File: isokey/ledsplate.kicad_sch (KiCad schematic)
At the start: 143 parts

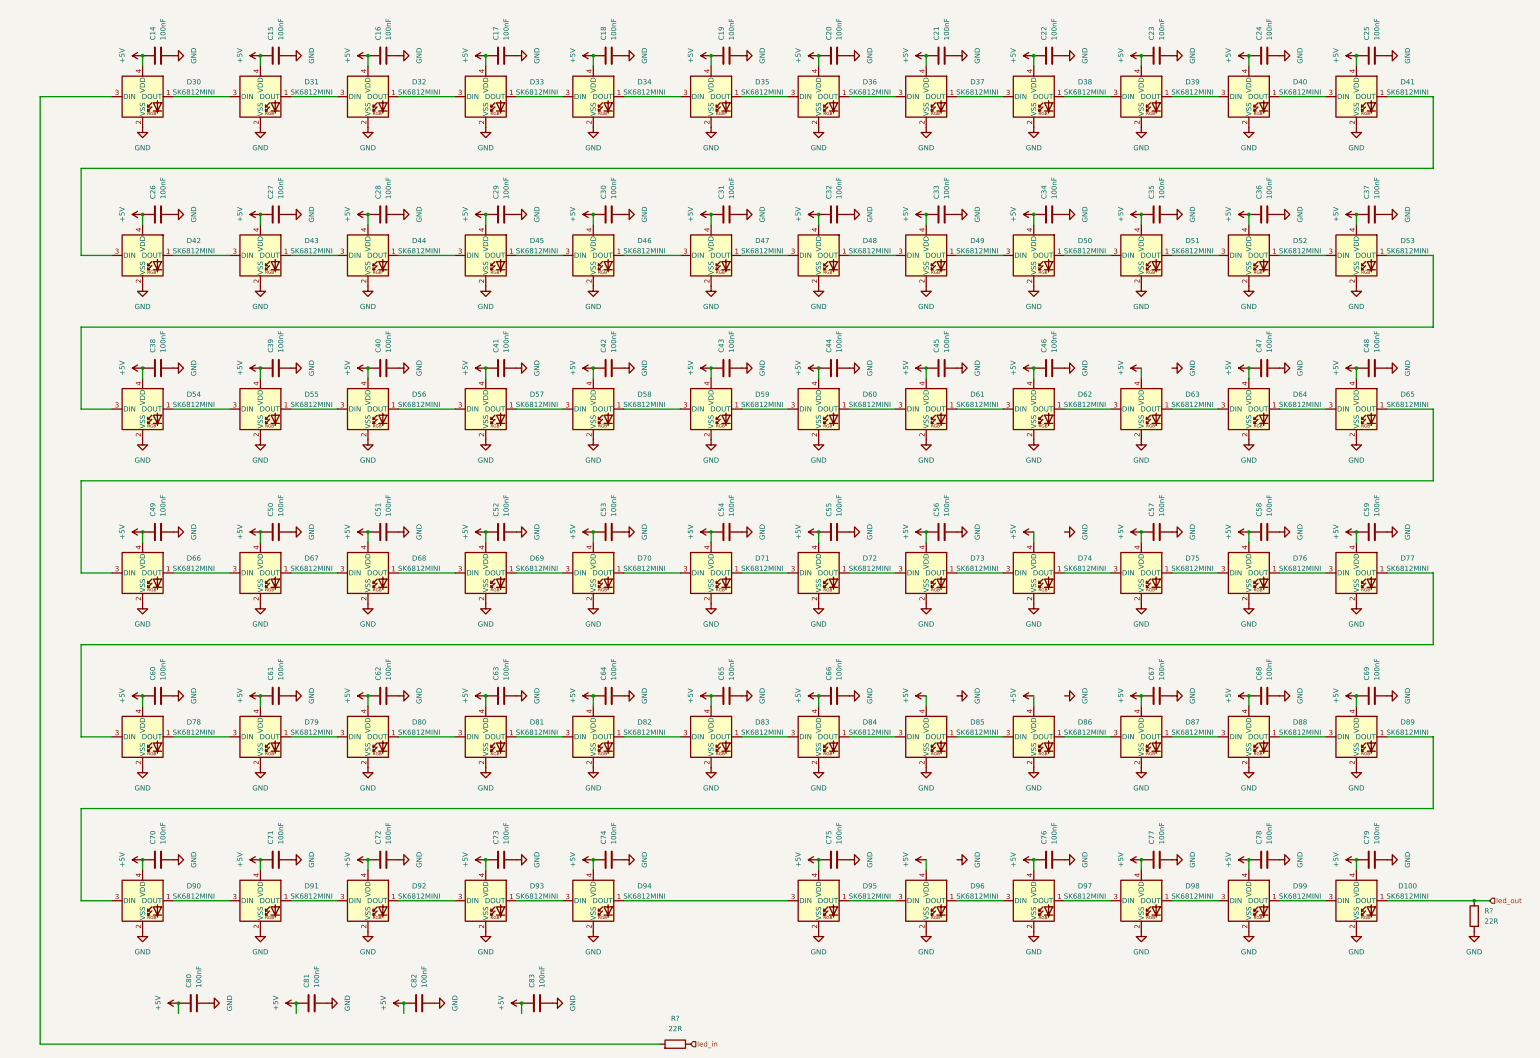
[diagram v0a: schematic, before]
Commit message: Continue routing
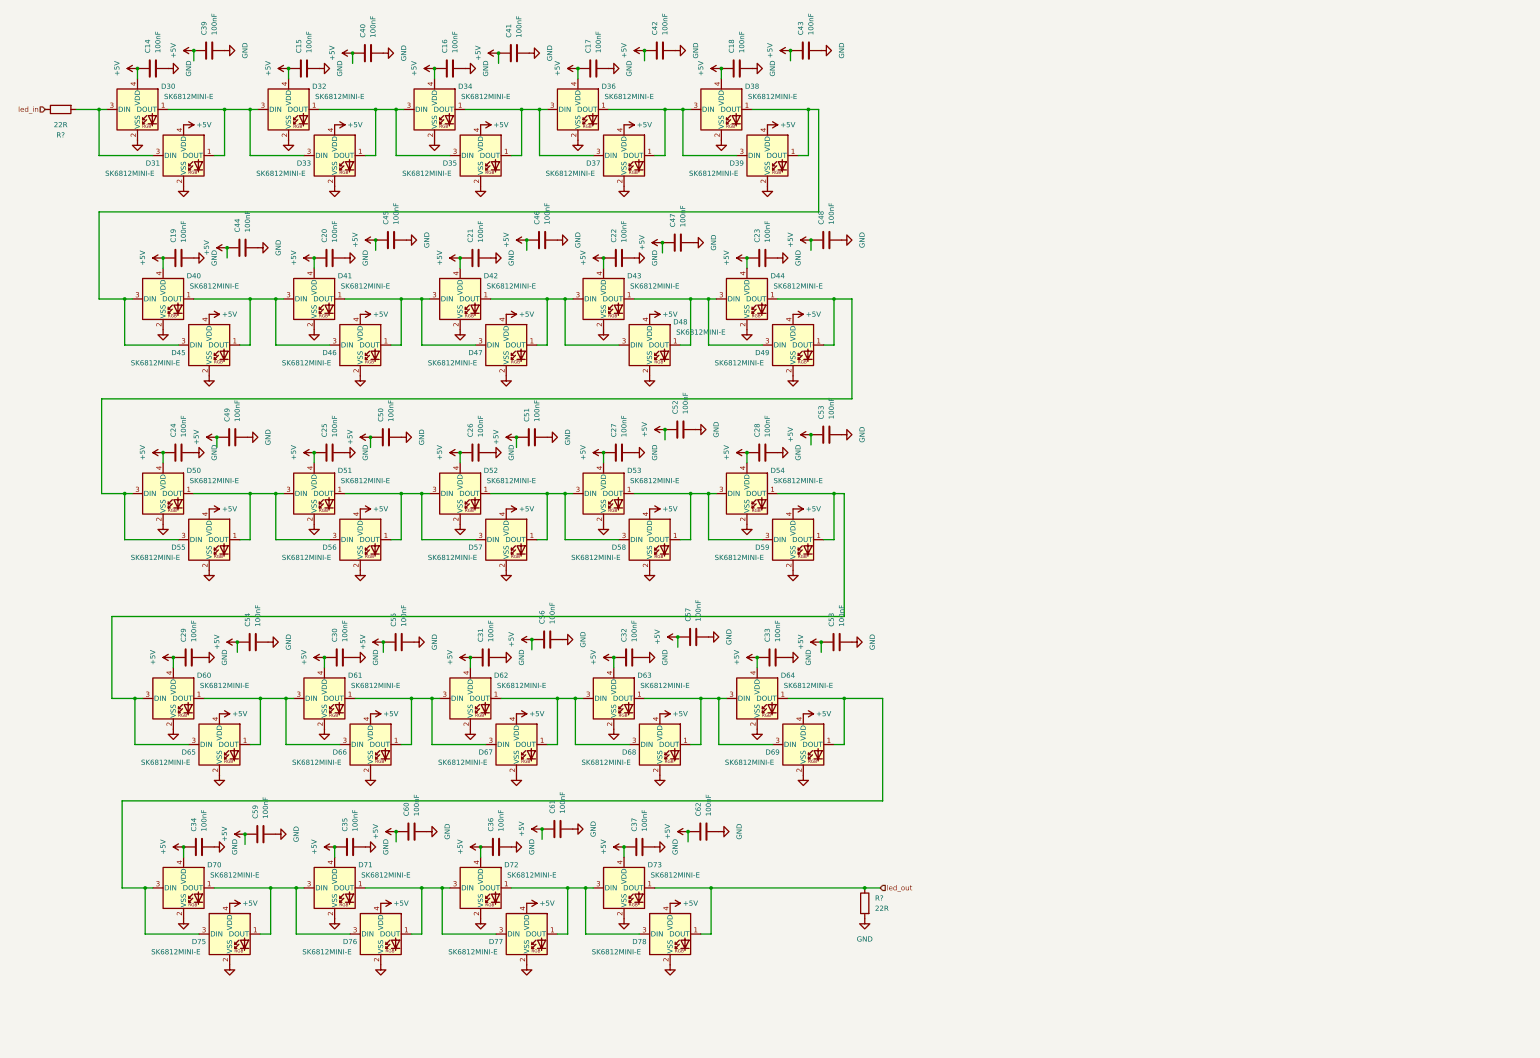
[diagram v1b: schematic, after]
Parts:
- removed C38, C63, C64, C65, C66, C67, C68, C69, C70, C71, C72, C73, C74, C75, C76, C77, C78, C79, C80, C81, C82, C83: 100nF, Capacitor_SMD:C_0603_1608Metric_Pad1.08x0.95mm_HandSolder, symbol Device:C
- removed D100, D74, D79, D80, D81, D82, D83, D84, D85, D86, D87, D88, D89, D90, D91, D92, D93, D94, D95, D96, D97, D98, D99: SK6812MINI, LED_SMD:LED_SK6812MINI_PLCC4_3.5x3.5mm_P1.75mm, symbol LED:SK6812MINI
- D30, D31, D32, D33, D34, D35, D36, D37, D38, D39, D40, D41, D42, D43, D44, D45, D46, D47, D48, D49, D50, D51, D52, D53, D54, D55, D56, D57, D58, D59, D60, D61, D62, D63, D64, D65, D66, D67, D68, D69, D70, D71, D72, D73, D75, D76, D77, D78: value SK6812MINI -> SK6812MINI-E
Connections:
- net led_out: now also D73.1 (DOUT), D78.1 (DOUT)
- net at D45.1 (DOUT), D46.3 (DIN): now also D40.1 (DOUT), D41.3 (DIN)
- net at D45.3 (DIN): now also D38.1 (DOUT), D39.1 (DOUT), D40.3 (DIN); no longer D44.1 (DOUT)
- net at D39.3 (DIN): now also D36.1 (DOUT), D37.1 (DOUT), D38.3 (DIN); no longer D38.1 (DOUT)
- net at D60.1 (DOUT), D61.3 (DIN): now also D65.1 (DOUT), D66.3 (DIN)
- net at D59.1 (DOUT), D60.3 (DIN): now also D54.1 (DOUT), D65.3 (DIN)
- net at D41.1 (DOUT), D42.3 (DIN): now also D46.1 (DOUT), D47.3 (DIN)
- net at D72.1 (DOUT), D73.3 (DIN): now also D77.1 (DOUT), D78.3 (DIN)
- net at D37.3 (DIN): now also D34.1 (DOUT), D35.1 (DOUT), D36.3 (DIN); no longer D36.1 (DOUT)
- net at D56.1 (DOUT), D57.3 (DIN): now also D51.1 (DOUT), D52.3 (DIN)
- net at D55.1 (DOUT), D56.3 (DIN): now also D50.1 (DOUT), D51.3 (DIN)
- net at D67.1 (DOUT), D68.3 (DIN): now also D62.1 (DOUT), D63.3 (DIN)
- net at D66.1 (DOUT), D67.3 (DIN): now also D61.1 (DOUT), D62.3 (DIN)
- net at D75.1 (DOUT), D76.3 (DIN): now also D70.1 (DOUT), D71.3 (DIN)
- net at D75.3 (DIN): now also D64.1 (DOUT), D69.1 (DOUT), D70.3 (DIN)
- net at D58.1 (DOUT), D59.3 (DIN): now also D53.1 (DOUT), D54.3 (DIN)
- net at D47.1 (DOUT), D48.3 (DIN): now also D42.1 (DOUT), D43.3 (DIN)
- net at D55.3 (DIN): now also D44.1 (DOUT), D49.1 (DOUT), D50.3 (DIN); no longer D54.1 (DOUT)
- net at D48.1 (DOUT), D49.3 (DIN): now also D43.1 (DOUT), D44.3 (DIN)
- net at D76.1 (DOUT), D77.3 (DIN): now also D71.1 (DOUT), D72.3 (DIN)
- net at D33.1 (DOUT), D34.3 (DIN): now also D32.1 (DOUT), D35.3 (DIN)
- net at D33.3 (DIN): now also D30.1 (DOUT), D31.1 (DOUT), D32.3 (DIN); no longer D32.1 (DOUT)
- net at D57.1 (DOUT), D58.3 (DIN): now also D52.1 (DOUT), D53.3 (DIN)
- net at D63.1 (DOUT), D64.3 (DIN): now also D68.1 (DOUT), D69.3 (DIN)
- net at D30.3 (DIN), R?.2: now also D31.3 (DIN)
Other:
- moved on the sheet: C14, D30, D31, R?
